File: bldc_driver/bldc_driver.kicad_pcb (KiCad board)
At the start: 2 copper layers, 46.4 x 26.5 mm, 81 parts, among them J1 I2C 1, J2 AVR-ISP-6, Q1 PSMN0R925YLC, Q2 PSMN0R925YLC, Q3 PSMN0R925YLC, Q4 PSMN0R925YLC, Q5 PSMN0R925YLC, Q6 PSMN0R925YLC, U1 ATmega328PB-AU, U2 INA199C2, U3 MIC4609

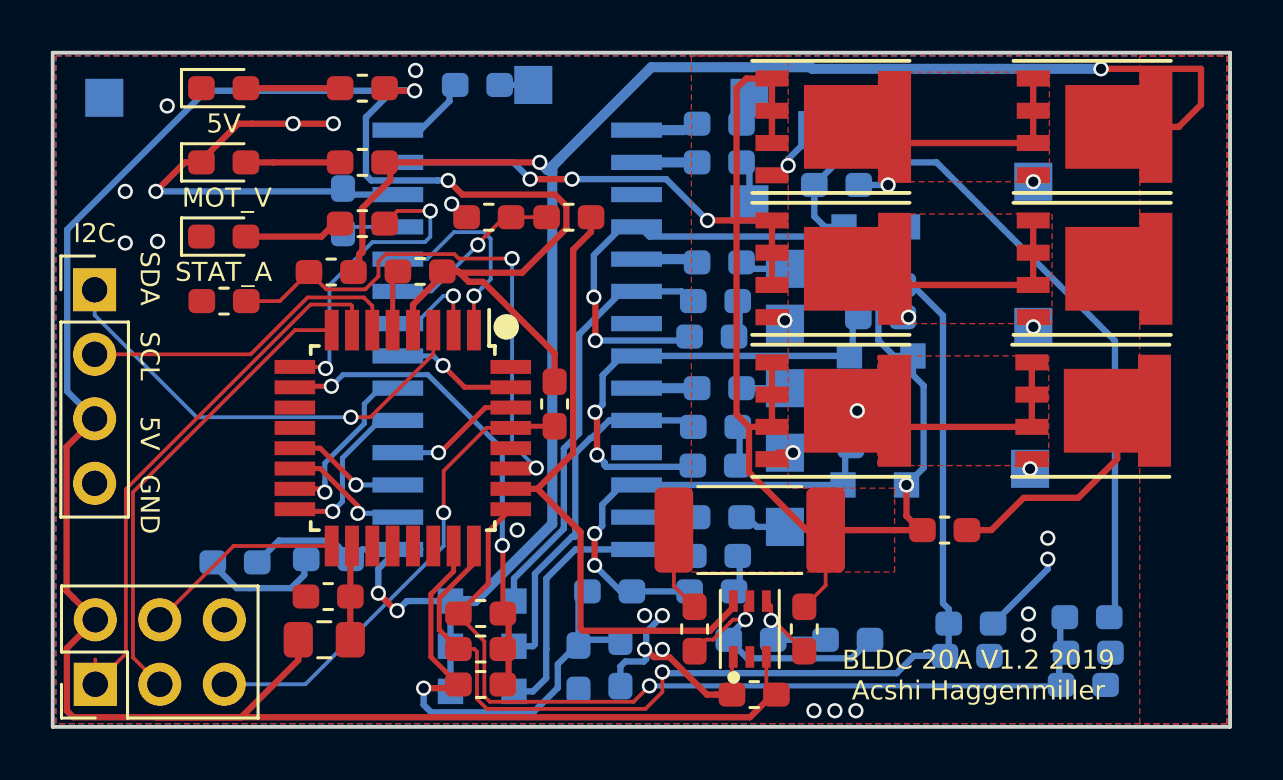
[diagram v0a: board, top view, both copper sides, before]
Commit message: added vias and things for grounding
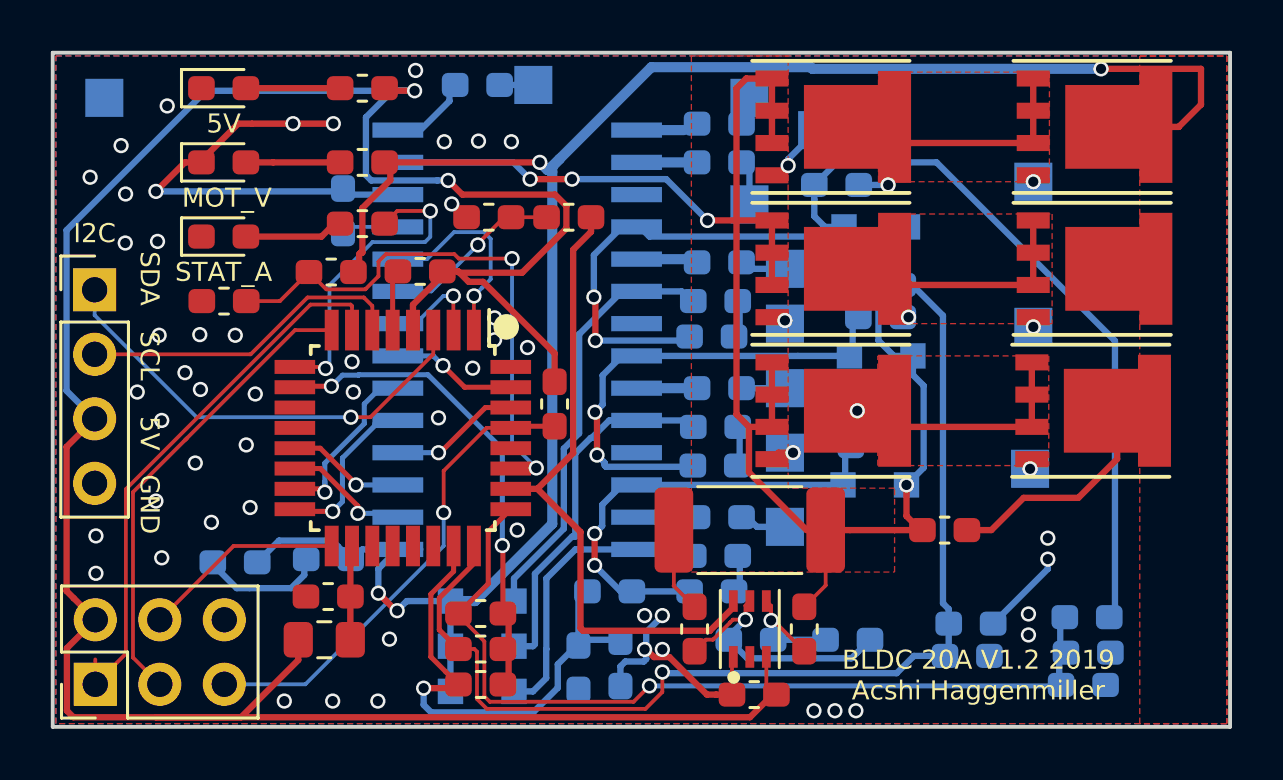
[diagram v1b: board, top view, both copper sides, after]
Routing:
- net GND: vias 21 -> 53
